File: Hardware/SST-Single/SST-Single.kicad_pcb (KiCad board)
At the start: 2 copper layers, 62 x 24 mm, 13 parts, among them J1 MJ-179PH, J2 Conn_01x03_Pin, J3 Conn_01x04_Pin, Q1 2SJ498-D, U1 FT231XS_Breakout, U2 LT1785AxN8

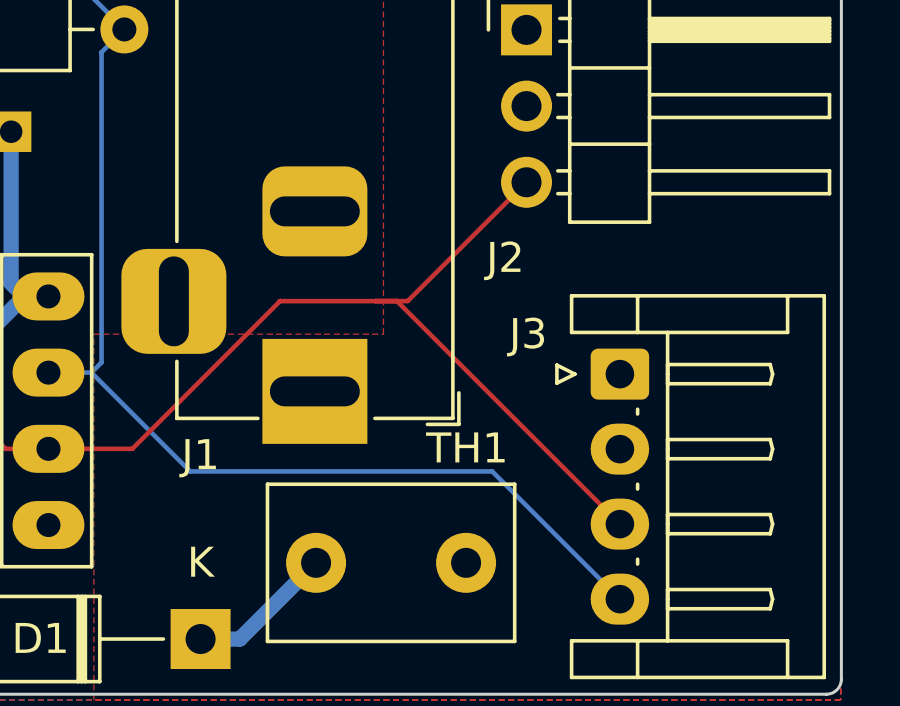
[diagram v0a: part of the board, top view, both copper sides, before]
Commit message: Update SST-Single Board
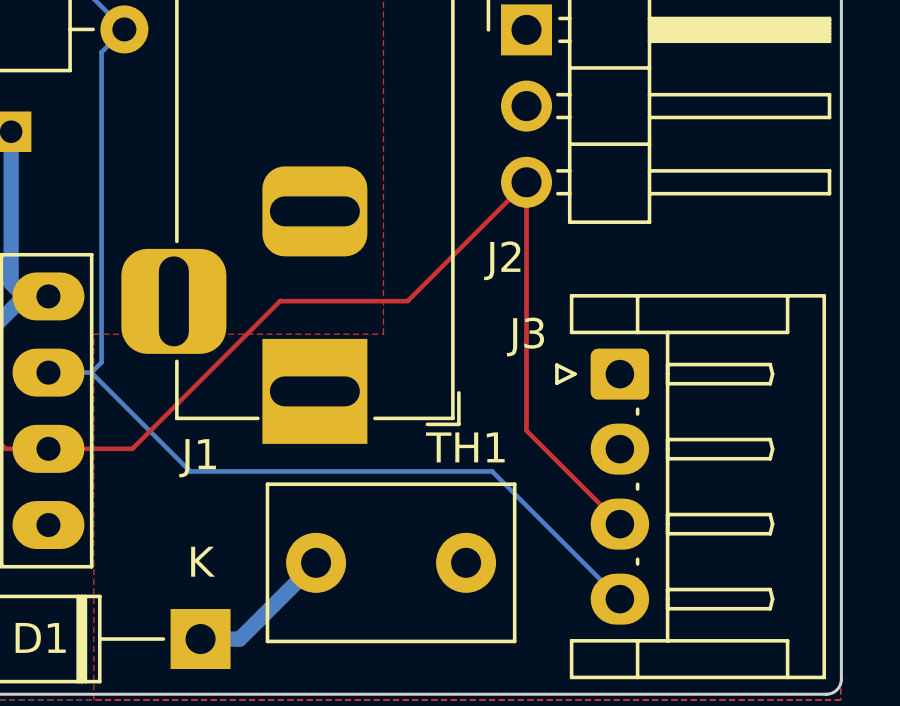
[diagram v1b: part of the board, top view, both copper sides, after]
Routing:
- net /RS485A: track 61.1 -> 62.6 mm
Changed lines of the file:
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@@
-	)
-	(segment
-		(start 147.5462 60.8938)
-		(end 146.4659 60.8938)
-		(width 0.1524)
-		(layer "F.Cu")
-		(net 9)
-	)
-	(segment
-		(start 146.4659 60.8938)
-		(end 147.1813 60.8938)
-		(width 0.1524)
-		(layer "F.Cu")
-		(net 9)
 	)
 	(segment
@@
 	)
 	(segment
-		(start 151.505 56.935)
-		(end 147.5462 60.8938)
+		(start 154.6175 68.33)
+		(end 151.505 65.2175)
 		(width 0.1524)
 		(layer "F.Cu")
@@
 	)
 	(segment
+		(start 151.505 65.2175)
+		(end 151.505 56.935)
+		(width 0.1524)
+		(layer "F.Cu")
+		(net 9)
+	)
+	(segment
 		(start 125.4 64.54)
 		(end 117.78 56.92)
@@
 	)
 	(segment
-		(start 135.57 65.82)
-		(end 134.1397 65.82)
+		(start 147.5462 60.8938)
+		(end 151.505 56.935)
 		(width 0.1524)
 		(layer "F.Cu")
@@
 	)
 	(segment
-		(start 146.4659 60.8938)
-		(end 143.2905 60.8938)
-		(width 0.1524)
-		(layer "F.Cu")
-		(net 9)
-	)
-	(segment
-		(start 147.1813 60.8938)
-		(end 154.6175 68.33)
+		(start 135.57 65.82)
+		(end 134.1397 65.82)
 		(width 0.1524)
 		(layer "F.Cu")
@@
 		(width 0.1524)
 		(layer "F.Cu")
+		(net 9)
+	)
+	(segment
+		(start 143.2905 60.8938)
+		(end 147.5462 60.8938)
+		(width 0.1524)
+		(layer "F.Cu")
